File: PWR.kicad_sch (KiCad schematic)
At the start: 35 parts, among them J1 USB_B_Mini, J15 Conn_01x02_Pin, J3 Conn_01x03_Pin, J7 Conn_01x02_Pin, Q1 AO3400A, Q2 AO3400A, U10 SRV05-4, U5 AMS1117-3.3

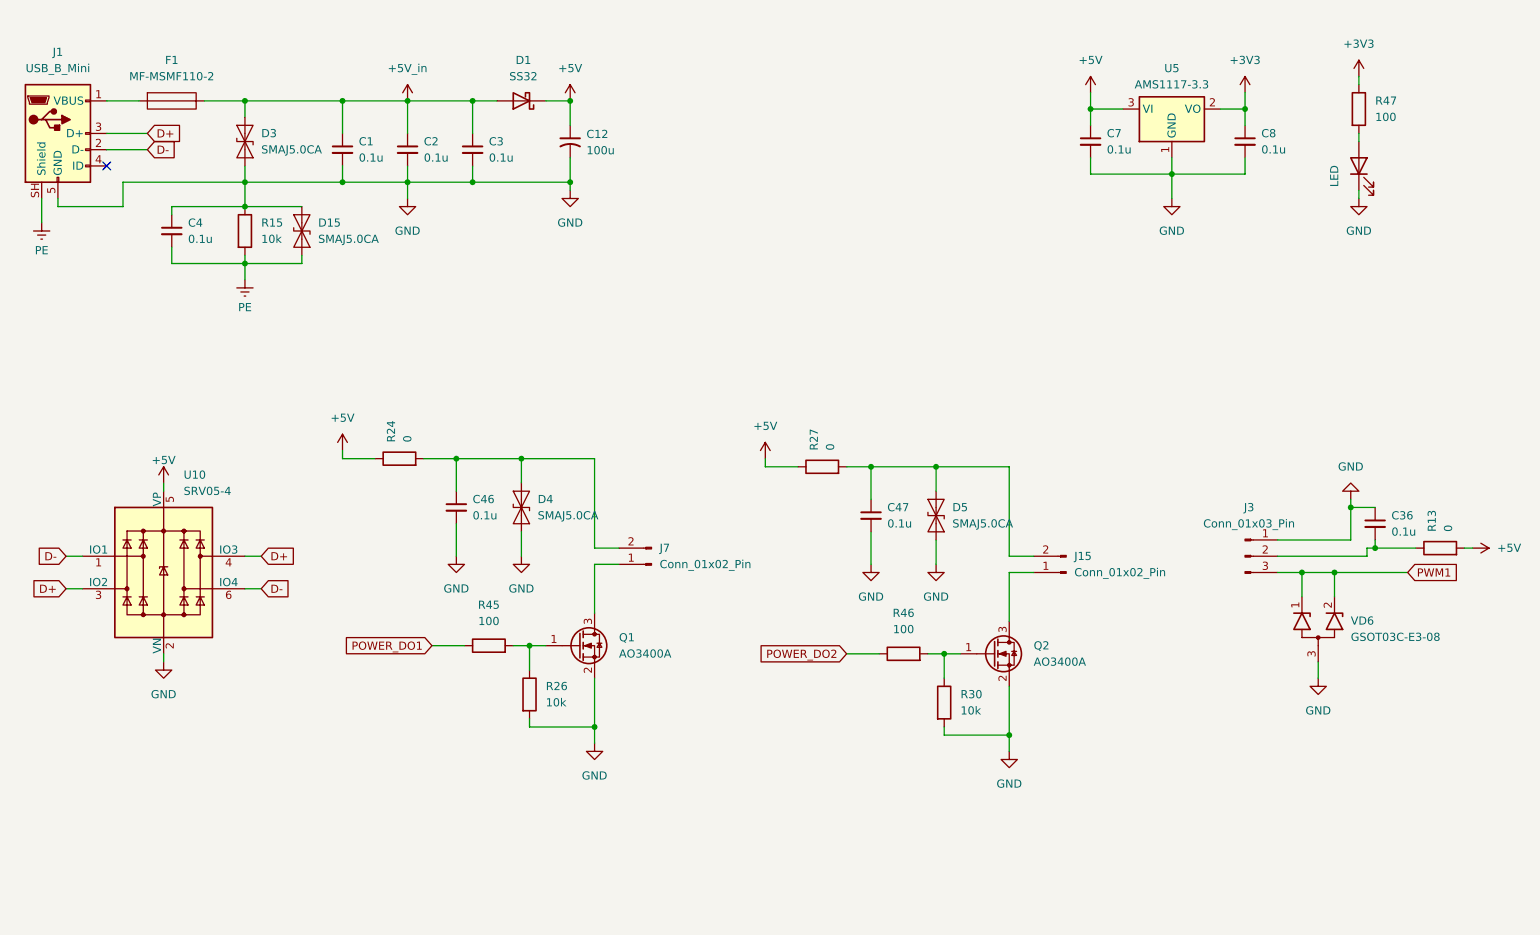
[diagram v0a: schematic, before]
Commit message: feat: добавлен дополнительный разъём для питания
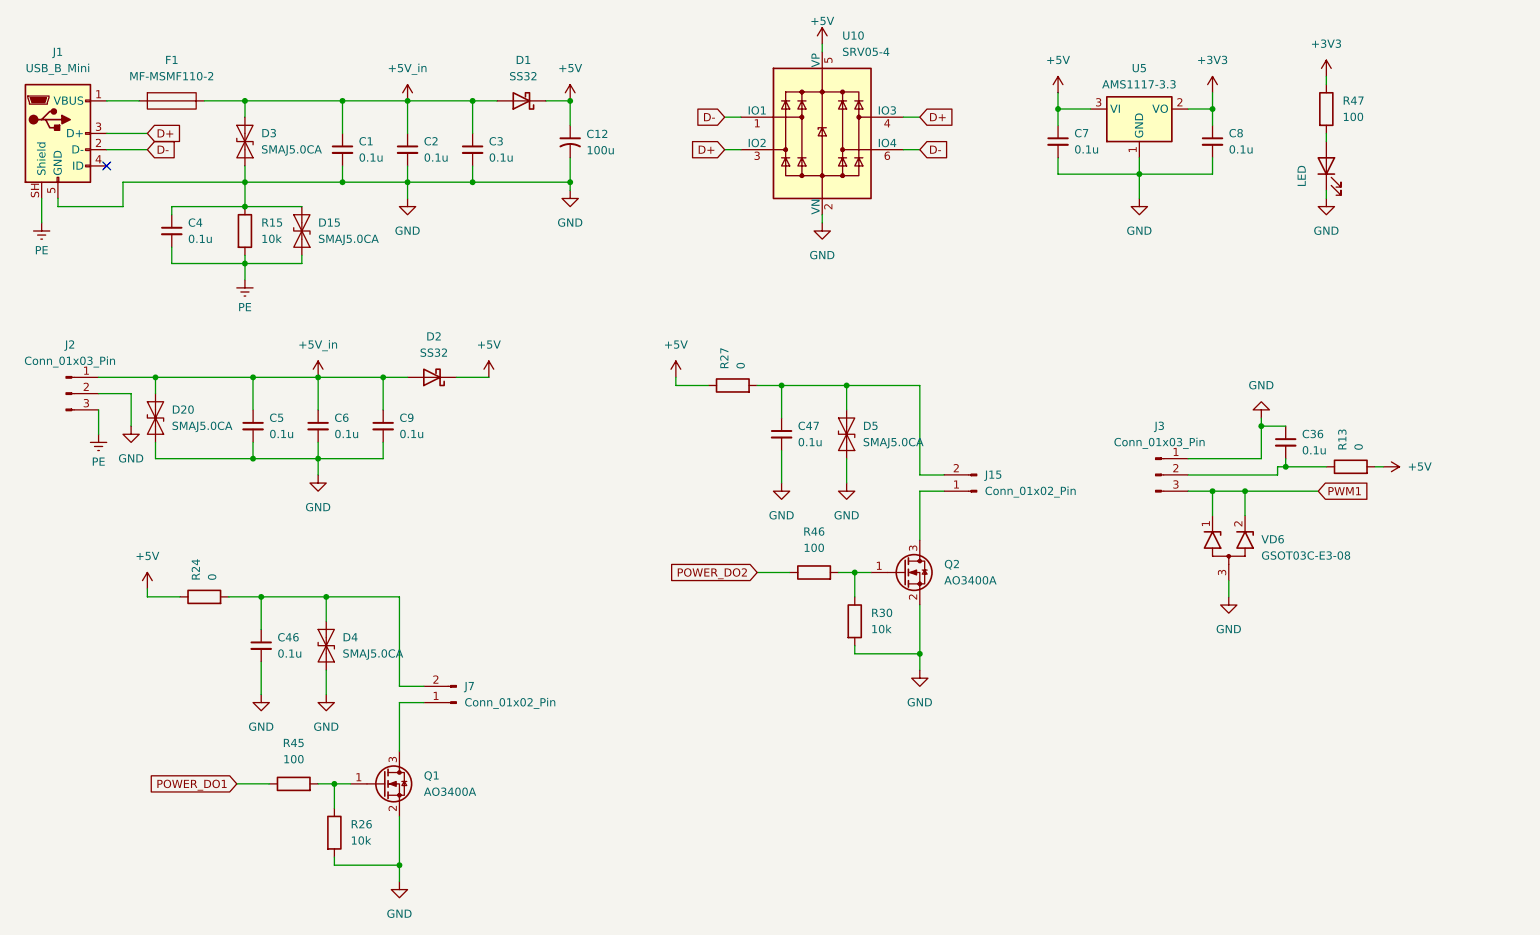
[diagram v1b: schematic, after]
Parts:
- added C5, C6, C9: 0.1u, Capacitor_SMD:C_0805_2012Metric_Pad1.18x1.45mm_HandSolder, symbol Device:C_Small
- added D2: SS32, Diode_SMD:D_SMA, symbol Diode:SS32
- added D20: SMAJ5.0CA, Diode_SMD:D_SMA, symbol Diode:SMAJ5.0CA
- added J2: Conn_01x03_Pin, Connector_JST:JST_NV_B03P-NV_1x03_P5.00mm_Vertical, symbol Connector:Conn_01x03_Pin
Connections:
- net +5V: now also D2.1 (K)
- net +5V_in: now also C5.1, C6.1, C9.1, D2.2 (A), D20.2 (A2), J2.1 (Pin_1)
- net GND: now also C5.2, C6.2, C9.2, D20.1 (A1), J2.2 (Pin_2)
- net PE: now also J2.3 (Pin_3)
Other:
- moved on the sheet: C36, C46, C47, C7, C8, D4, D5, J15, J3, J7, Q1, Q2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
